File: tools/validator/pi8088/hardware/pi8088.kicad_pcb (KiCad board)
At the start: 2 copper layers, 31 x 52 mm, 2 parts

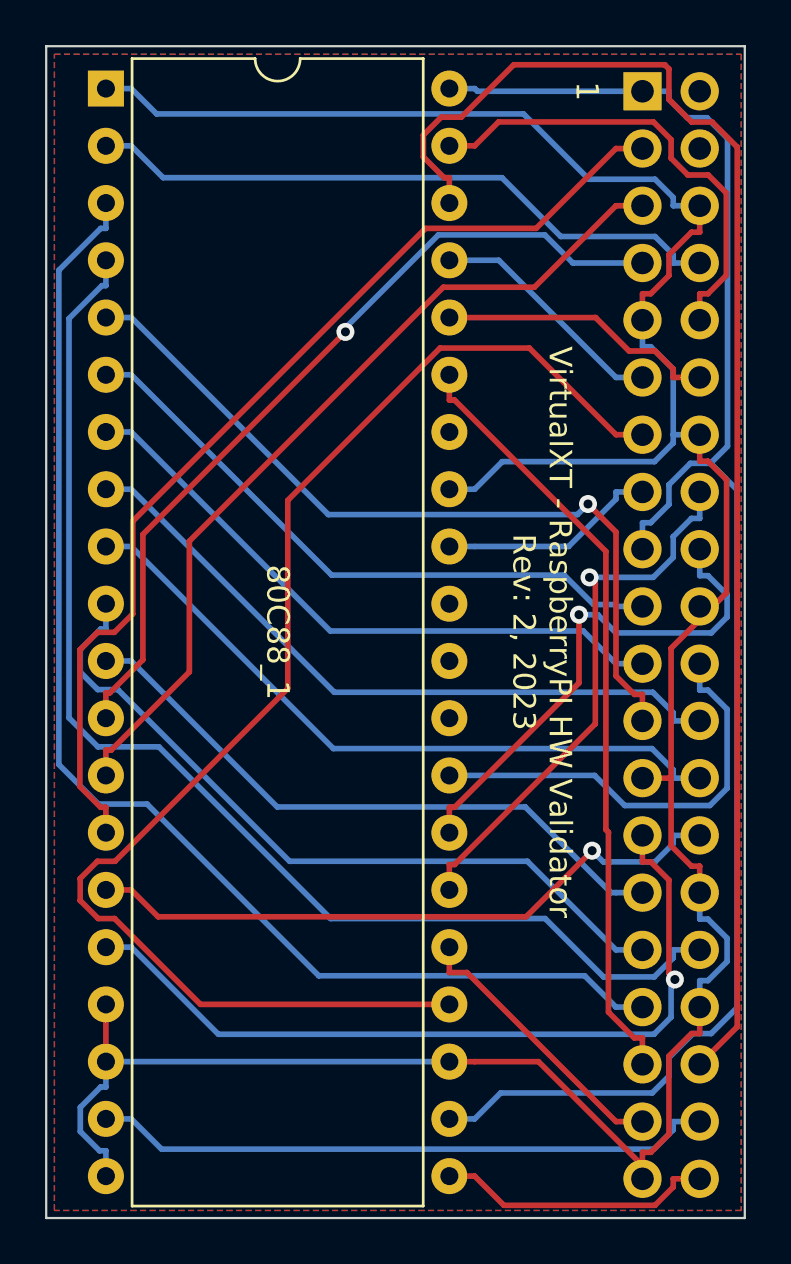
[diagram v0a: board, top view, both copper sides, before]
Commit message: Added r1 validator
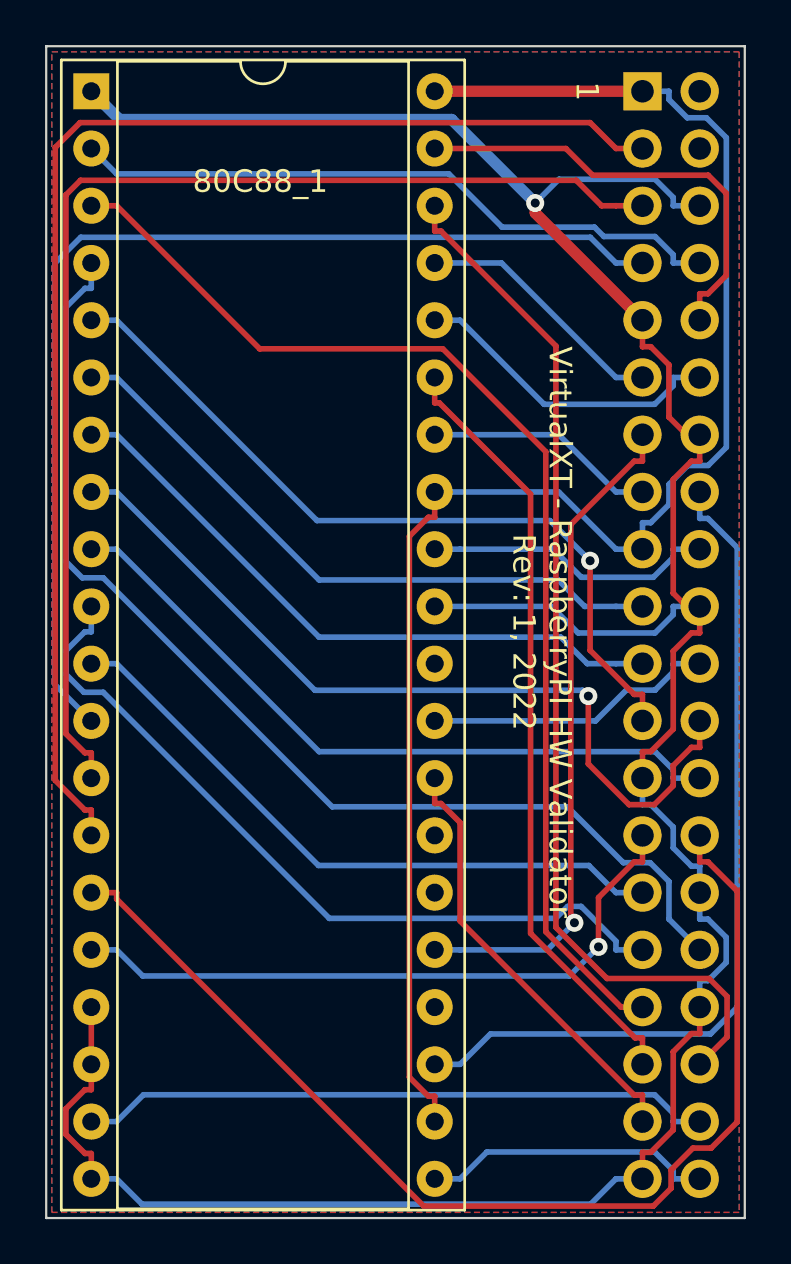
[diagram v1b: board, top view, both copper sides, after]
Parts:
- 80C88_1: value 8088_Max_Mode -> 8088_Min_Mode; footprint Package_DIP:DIP-40_W15.24mm -> Package_DIP:DIP-40_W15.24mm_Socket
- moved 80C88_1 0.66 mm to (120.0, 56.0)
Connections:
- 80C88_1 pad 23: Net-(80C88_1-Pad1) -> Net-(80C88_1-Pad23)
- 80C88_1 pad 24: Net-(GPIO_1-Pad13) -> unconnected-(80C88_1-Pad24)
- 80C88_1 pad 25: Net-(GPIO_1-Pad37) -> Net-(80C88_1-Pad25)
- 80C88_1 pad 26: Net-(GPIO_1-Pad16) -> unconnected-(80C88_1-Pad26)
- 80C88_1 pad 27: Net-(GPIO_1-Pad18) -> unconnected-(80C88_1-Pad27)
- 80C88_1 pad 28: Net-(GPIO_1-Pad22) -> Net-(80C88_1-Pad28)
- 80C88_1 pad 29: unconnected-(80C88_1-Pad29) -> Net-(80C88_1-Pad29)
- 80C88_1 pad 31: unconnected-(80C88_1-Pad31) -> Net-(80C88_1-Pad1)
- 80C88_1 pad 32: Net-(GPIO_1-Pad15) -> Net-(80C88_1-Pad32)
- 80C88_1 pad 33: Net-(80C88_1-Pad1) -> Net-(80C88_1-Pad22)
- 80C88_1 pad 34: unconnected-(80C88_1-Pad34) -> Net-(80C88_1-Pad34)
- GPIO_1 pad 13: Net-(GPIO_1-Pad13) -> Net-(80C88_1-Pad25)
- GPIO_1 pad 15: Net-(GPIO_1-Pad15) -> Net-(80C88_1-Pad34)
- GPIO_1 pad 16: Net-(GPIO_1-Pad16) -> Net-(80C88_1-Pad23)
- GPIO_1 pad 18: Net-(GPIO_1-Pad18) -> Net-(80C88_1-Pad32)
- GPIO_1 pad 22: Net-(GPIO_1-Pad22) -> Net-(80C88_1-Pad29)
- GPIO_1 pad 37: Net-(GPIO_1-Pad37) -> Net-(80C88_1-Pad28)
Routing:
- net Net-(GPIO_1-Pad13): track 60.5 -> 0.00 mm
- net Net-(80C88_1-Pad23): track 0.00 -> 38.2 mm
- net Net-(80C88_1-Pad25): track 0.00 -> 30.0 mm, vias 0 -> 1
- net Net-(GPIO_1-Pad16): track 24.5 -> 0.00 mm, vias 1 -> 0
- net Net-(GPIO_1-Pad18): track 23.1 -> 0.00 mm, vias 1 -> 0
- net Net-(80C88_1-Pad15): track 29.0 -> 50.2 mm, vias 1 -> 0
- net Net-(GPIO_1-Pad22): track 19.4 -> 0.00 mm
- net Net-(80C88_1-Pad28): track 0.00 -> 19.4 mm
- net Net-(80C88_1-Pad38): track 62.5 -> 46.8 mm
- net Net-(80C88_1-Pad13): track 38.3 -> 52.8 mm
- net Net-(80C88_1-Pad29): track 0.00 -> 13.0 mm
- net Net-(80C88_1-Pad14): track 45.3 -> 58.3 mm
- net Net-(80C88_1-Pad32): track 0.00 -> 13.0 mm
- net Net-(GPIO_1-Pad37): track 12.4 -> 0.00 mm
- net Net-(80C88_1-Pad12): track 37.2 -> 48.0 mm, vias 1 -> 0
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- added copper zone on B.Cu, net Net-(80C88_1-Pad1)
- removed copper zone on B.Cu, net Net-(80C88_1-Pad22)
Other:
- board text added: "VirtualXT - RaspberryPI HW Validator Rev: 1, 2022"
- board text removed: "VirtualXT - RaspberryPI HW Validator Rev: 2, 2023"

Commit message: New pcb design
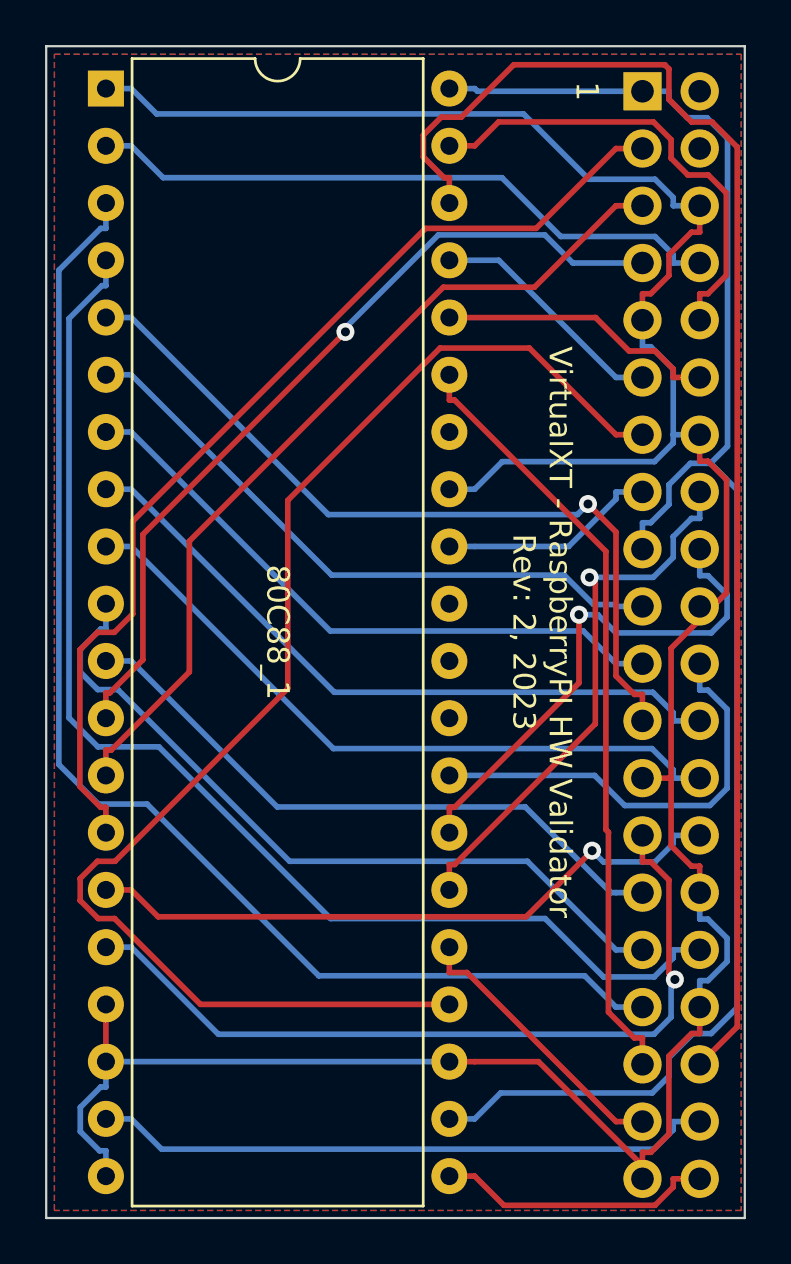
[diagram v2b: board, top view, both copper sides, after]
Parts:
- 80C88_1: value 8088_Min_Mode -> 8088_Max_Mode; footprint Package_DIP:DIP-40_W15.24mm_Socket -> Package_DIP:DIP-40_W15.24mm
- moved 80C88_1 0.66 mm to (120.7, 55.9)
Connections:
- 80C88_1 pad 23: Net-(80C88_1-Pad23) -> Net-(80C88_1-Pad1)
- 80C88_1 pad 24: unconnected-(80C88_1-Pad24) -> Net-(GPIO_1-Pad13)
- 80C88_1 pad 25: Net-(80C88_1-Pad25) -> Net-(GPIO_1-Pad37)
- 80C88_1 pad 26: unconnected-(80C88_1-Pad26) -> Net-(GPIO_1-Pad16)
- 80C88_1 pad 27: unconnected-(80C88_1-Pad27) -> Net-(GPIO_1-Pad18)
- 80C88_1 pad 28: Net-(80C88_1-Pad28) -> Net-(GPIO_1-Pad22)
- 80C88_1 pad 29: Net-(80C88_1-Pad29) -> unconnected-(80C88_1-Pad29)
- 80C88_1 pad 31: Net-(80C88_1-Pad1) -> unconnected-(80C88_1-Pad31)
- 80C88_1 pad 32: Net-(80C88_1-Pad32) -> Net-(GPIO_1-Pad15)
- 80C88_1 pad 33: Net-(80C88_1-Pad22) -> Net-(80C88_1-Pad1)
- 80C88_1 pad 34: Net-(80C88_1-Pad34) -> unconnected-(80C88_1-Pad34)
- GPIO_1 pad 13: Net-(80C88_1-Pad25) -> Net-(GPIO_1-Pad13)
- GPIO_1 pad 15: Net-(80C88_1-Pad34) -> Net-(GPIO_1-Pad15)
- GPIO_1 pad 16: Net-(80C88_1-Pad23) -> Net-(GPIO_1-Pad16)
- GPIO_1 pad 18: Net-(80C88_1-Pad32) -> Net-(GPIO_1-Pad18)
- GPIO_1 pad 22: Net-(80C88_1-Pad29) -> Net-(GPIO_1-Pad22)
- GPIO_1 pad 37: Net-(80C88_1-Pad28) -> Net-(GPIO_1-Pad37)
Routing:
- net Net-(GPIO_1-Pad13): track 0.00 -> 60.5 mm
- net Net-(80C88_1-Pad23): track 38.2 -> 0.00 mm
- net Net-(80C88_1-Pad25): track 30.0 -> 0.00 mm, vias 1 -> 0
- net Net-(GPIO_1-Pad16): track 0.00 -> 24.5 mm, vias 0 -> 1
- net Net-(GPIO_1-Pad18): track 0.00 -> 23.1 mm, vias 0 -> 1
- net Net-(80C88_1-Pad15): track 50.2 -> 29.0 mm, vias 0 -> 1
- net Net-(GPIO_1-Pad22): track 0.00 -> 19.4 mm
- net Net-(80C88_1-Pad28): track 19.4 -> 0.00 mm
- net Net-(80C88_1-Pad38): track 46.8 -> 62.5 mm
- net Net-(80C88_1-Pad13): track 52.8 -> 38.3 mm
- net Net-(80C88_1-Pad29): track 13.0 -> 0.00 mm
- net Net-(80C88_1-Pad14): track 58.3 -> 45.3 mm
- net Net-(80C88_1-Pad32): track 13.0 -> 0.00 mm
- net Net-(GPIO_1-Pad37): track 0.00 -> 12.4 mm
- net Net-(80C88_1-Pad12): track 48.0 -> 37.2 mm, vias 0 -> 1
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- added copper zone on B.Cu, net Net-(80C88_1-Pad22)
- removed copper zone on B.Cu, net Net-(80C88_1-Pad1)
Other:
- board text added: "VirtualXT - RaspberryPI HW Validator Rev: 2, 2023"
- board text removed: "VirtualXT - RaspberryPI HW Validator Rev: 1, 2022"
